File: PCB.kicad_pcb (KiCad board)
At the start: 2 copper layers, 150 x 150 mm, 14 parts

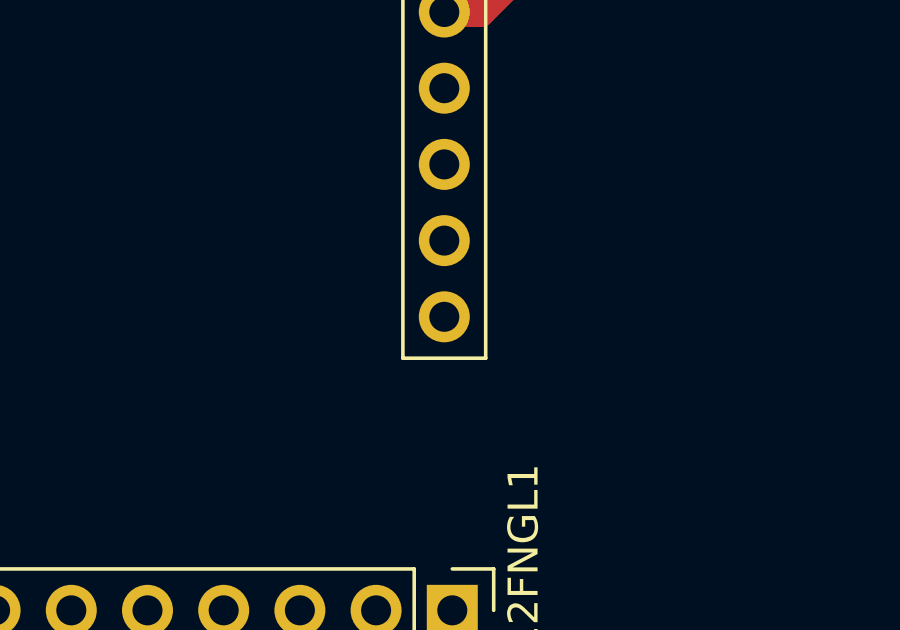
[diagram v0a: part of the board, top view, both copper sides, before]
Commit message: 2
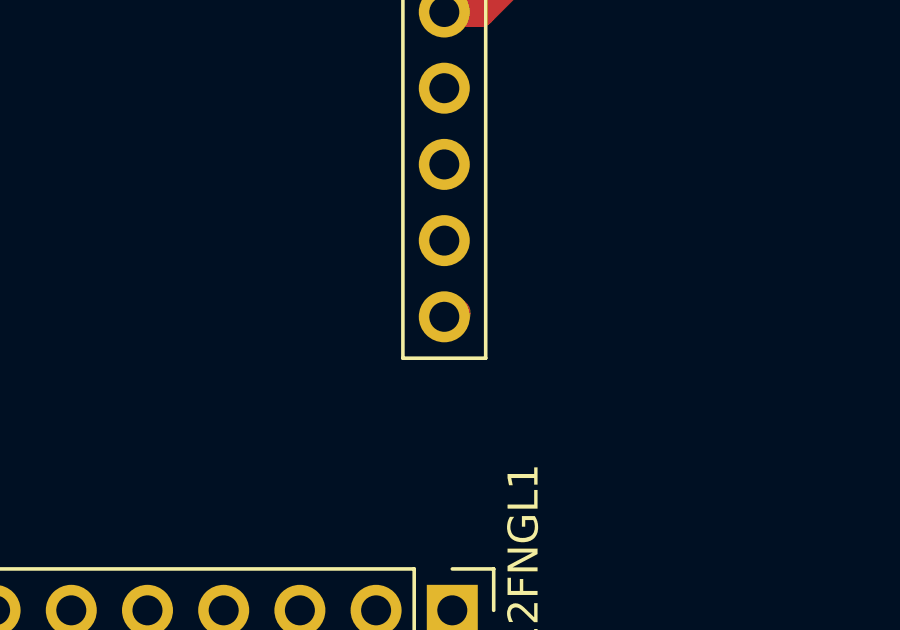
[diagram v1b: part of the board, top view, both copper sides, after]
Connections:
- PicoR1 pad 3: unconnected-(PicoR1-Pin_3-Pad3) -> GND1
- TB6612FNGL1 pad 1: GND -> GND1
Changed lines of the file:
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@@
 	(net 40 "unconnected-(PicoR1-Pin_10-Pad10)")
 	(net 41 "unconnected-(PicoR1-Pin_18-Pad18)")
-	(net 42 "unconnected-(PicoR1-Pin_3-Pad3)")
+	(net 42 "GND1")
 	(net 43 "Net-(PicoR1-Pin_1)")
 	(net 44 "Net-(PicoR1-Pin_7)")
@@
 			(layers "*.Cu" "*.Mask")
 			(remove_unused_layers no)
-			(net 42 "unconnected-(PicoR1-Pin_3-Pad3)")
+			(net 42 "GND1")
 			(pinfunction "Pin_3")
 			(pintype "passive")
@@
 			(layers "*.Cu" "*.Mask")
 			(remove_unused_layers no)
-			(net 2 "GND")
+			(net 42 "GND1")
 			(pinfunction "Pin_1")
 			(pintype "passive")
@@
 	)
 	(segment
+		(start 139.62 112.120293)
+		(end 139.879707 112.120293)
+		(width 1)
+		(layer "F.Cu")
+		(net 36)
+	)
+	(segment
+		(start 139.879707 112.120293)
+		(end 140 112)
+		(width 1)
+		(layer "F.Cu")
+		(net 36)
+	)
+	(segment
